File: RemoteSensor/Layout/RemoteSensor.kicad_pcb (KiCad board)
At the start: 2 copper layers, 50.8 x 50.8 mm, 70 parts, among them J1 USB_B_Micro, J2 BATT_CONN, J3 LCD_HEADER, Q1 Si3443DV, Q2 2N7002, Q3 2N7002, Q6 2N7002, SW1 BTN_RST, SW2 FLASH, SW3 SW_Push, SW4 SW_Push, SW5 SW_Push, U1 MCP73831-2-OT, U10 FT231XS, U3 BD48ExxG, U4 BD48ExxG, U5 LM3671MF, U6 74LVC2G02, U7 ESP-12F, U8 ds7505s+, U9 MCP23008-E_P

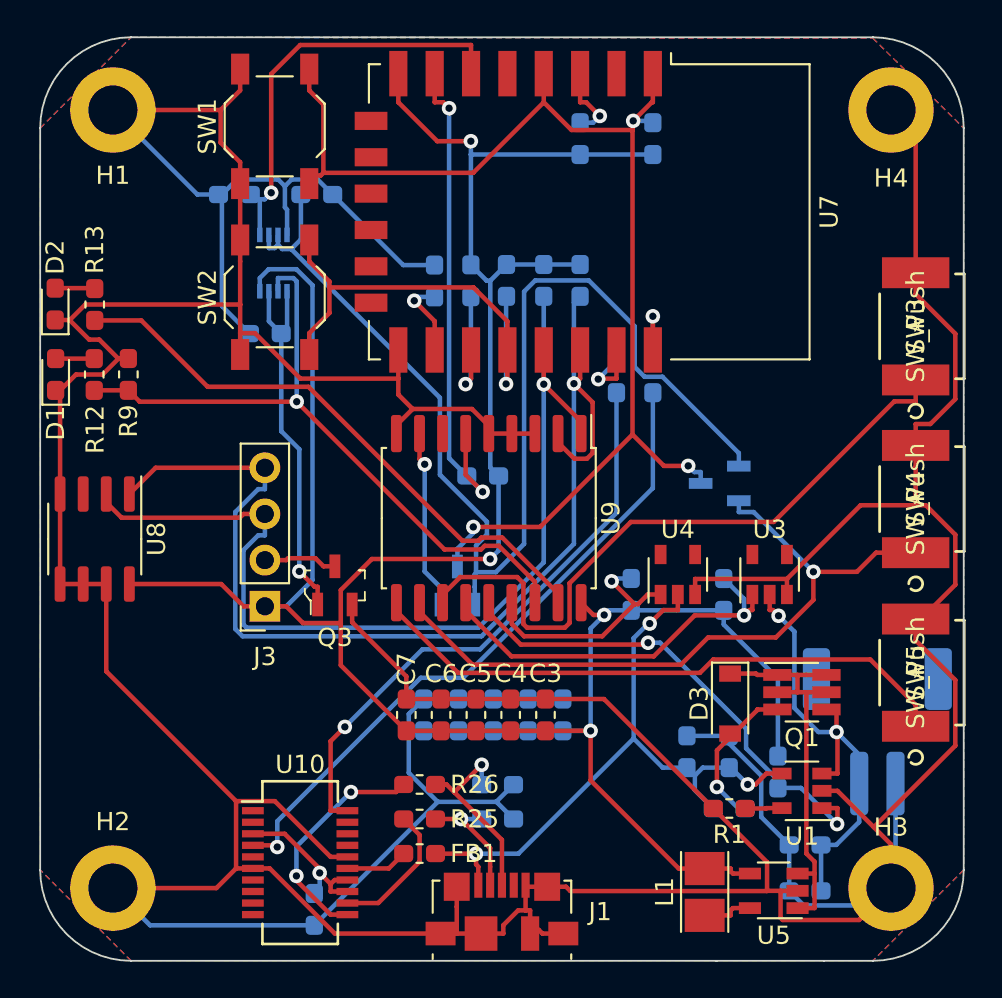
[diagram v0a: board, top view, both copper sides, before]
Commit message: Layout
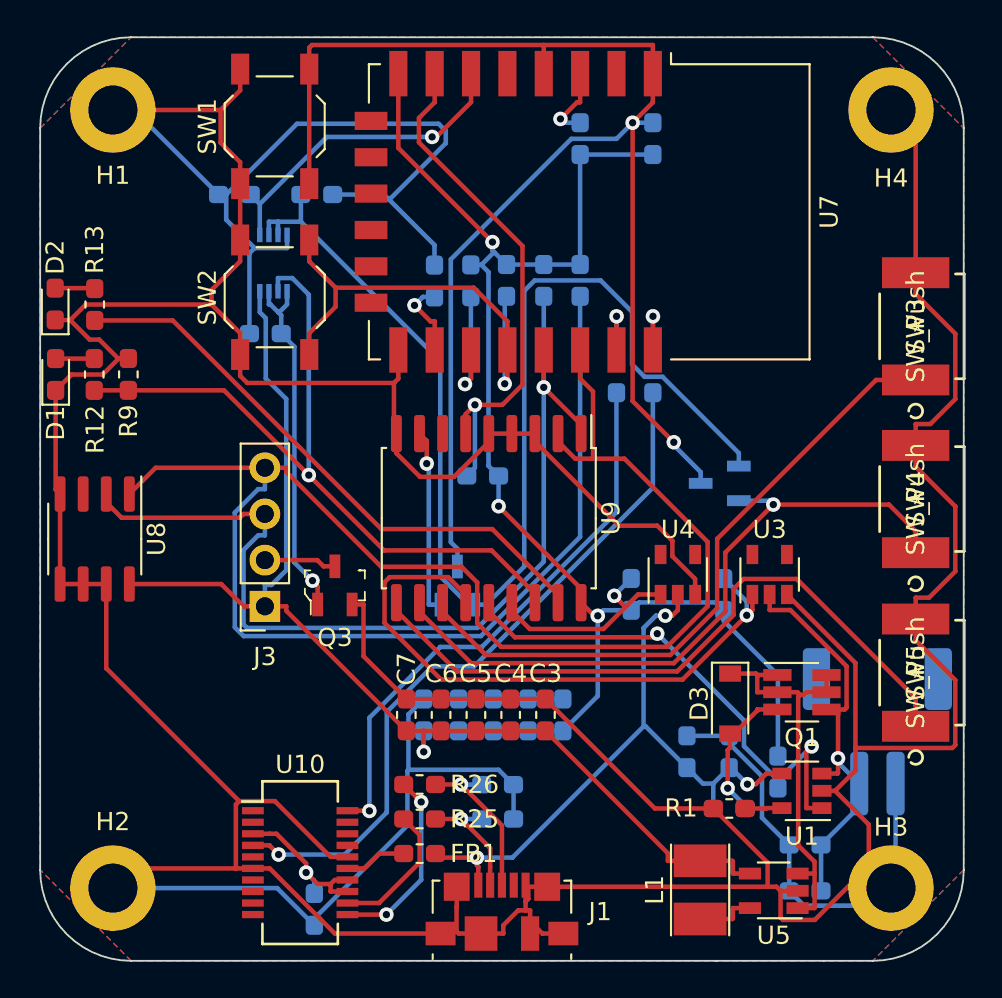
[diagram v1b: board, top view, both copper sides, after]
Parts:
- L1: footprint Inductor_SMD:L_Taiyo-Yuden_NR-24xx_HandSoldering -> Inductor_SMD:L_Taiyo-Yuden_NR-30xx_HandSoldering
- moved L1 0.27 mm to (183.3, 137.9)
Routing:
- net /Processor/SDA: track 61.6 -> 104.0 mm, vias 1 -> 0
- net GND: track 360.7 -> 386.6 mm
- net RST: track 68.2 -> 85.4 mm, vias 3 -> 2
- net 3.3V: track 157.2 -> 144.6 mm
- net BATT_STS: track 21.6 -> 34.2 mm
- net SLEEP_PIN: track 23.1 -> 17.9 mm
- net DOWN_BTN: track 33.0 -> 37.6 mm
- net HB_PIN: track 38.4 -> 42.1 mm
- net PRG_RX: track 36.3 -> 39.0 mm
- net V_BATT: track 25.3 -> 22.9 mm, vias 2 -> 1
- net Net-(R26-Pad1): track 12.8 -> 10.5 mm
- net SLEEP_STS: track 65.4 -> 67.2 mm
- net USBDP: track 10.6 -> 9.02 mm
- net CHARGER_STS: track 13.5 -> 12.0 mm
- net CHARGE_STS: track 27.2 -> 28.6 mm
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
